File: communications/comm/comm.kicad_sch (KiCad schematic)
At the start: 2 parts, among them J1 Conn_Coaxial, U1 SX1276

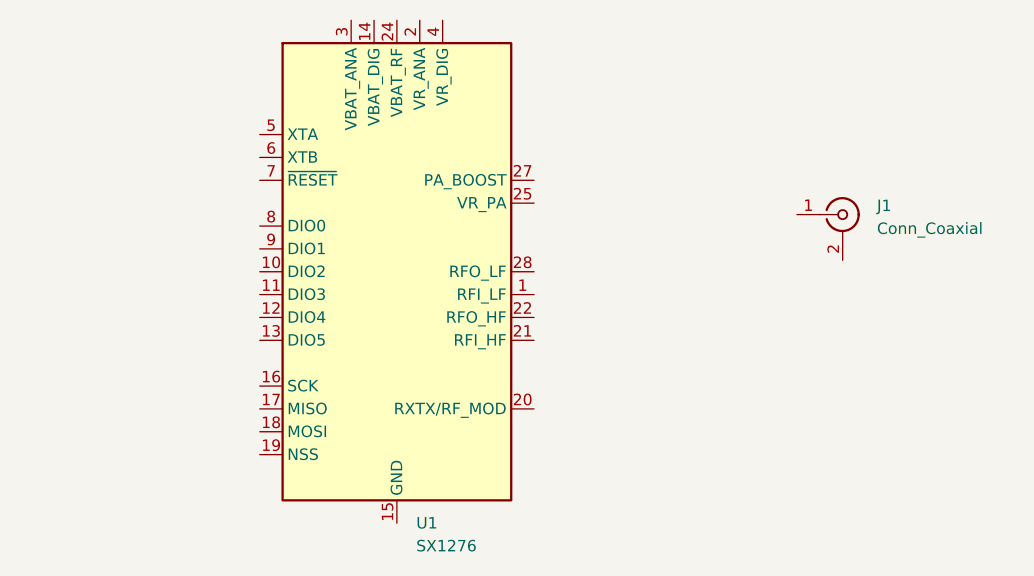
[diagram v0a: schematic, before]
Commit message: refresh
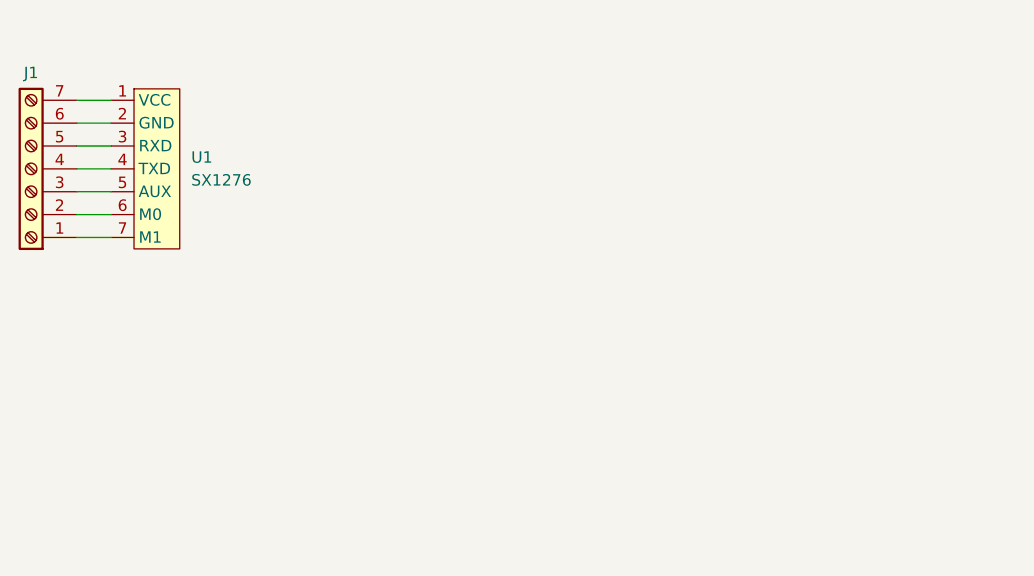
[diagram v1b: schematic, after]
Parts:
- removed J1: Conn_Coaxial, Connector_Coaxial:SMA_Molex_73251-1153_EdgeMount_Horizontal, symbol Connector:Conn_Coaxial
- removed U1: SX1276, Package_DFN_QFN:QFN-28-1EP_6x6mm_P0.65mm_EP4.8x4.8mm, symbol RF:SX1276
- added J1: Screw_Terminal_01x07, Connector_JST:JST_EH_B7B-EH-A_1x07_P2.50mm_Vertical, symbol Connector:Screw_Terminal_01x07
- added U1: SX1276, Connector_PinHeader_2.54mm:PinHeader_1x07_P2.54mm_Vertical, symbol me:SX1276-module
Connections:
- new net: J1.1 (Pin_1), U1.7 (M1)
- new net: J1.2 (Pin_2), U1.6 (M0)
- new net: J1.3 (Pin_3), U1.5 (AUX)
- new net: J1.4 (Pin_4), U1.4 (TXD)
- new net: J1.5 (Pin_5), U1.3 (RXD)
- new net: J1.6 (Pin_6), U1.2 (GND)
- new net: J1.7 (Pin_7), U1.1 (VCC)
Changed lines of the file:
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@@
 	(generator_version "9.0")
 	(paper "A4")
+	(wire
+		(pts
+			(xy 99.06 77.47) (xy 95.25 77.47)
+		)
+		(stroke
+			(width 0)
+			(type default)
+		)
+	)
+	(wire
+		(pts
+			(xy 99.06 87.63) (xy 95.25 87.63)
+		)
+		(stroke
+			(width 0)
+			(type default)
+		)
+	)
+	(wire
+		(pts
+			(xy 99.06 85.09) (xy 95.25 85.09)
+		)
+		(stroke
+			(width 0)
+			(type default)
+		)
+	)
+	(wire
+		(pts
+			(xy 99.06 82.55) (xy 95.25 82.55)
+		)
+		(stroke
+			(width 0)
+			(type default)
+		)
+	)
+	(wire
+		(pts
+			(xy 99.06 90.17) (xy 95.25 90.17)
+		)
+		(stroke
+			(width 0)
+			(type default)
+		)
+	)
+	(wire
+		(pts
+			(xy 99.06 80.01) (xy 95.25 80.01)
+		)
+		(stroke
+			(width 0)
+			(type default)
+		)
+	)
+	(wire
+		(pts
+			(xy 99.06 74.93) (xy 95.25 74.93)
+		)
+		(stroke
+			(width 0)
+			(type default)
+		)
+	)
 	(symbol
-		(lib_id "Connector:Conn_Coaxial")
-		(at 180.34 87.63 0)
+		(lib_id "Connector:Screw_Terminal_01x07")
+		(at 90.17 82.55 180)
 		(unit 1)
 		(exclude_from_sim no)
@@
 		(on_board yes)
 		(dnp no)
-		(fields_autoplaced yes)
 		(property "Reference" "J1"
-			(at 184.15 86.6531 0)
-			(effects
-				(font
-					(size 1.27 1.27)
-				)
-				(justify left)
-			)
-		)
-		(property "Value" "Conn_Coaxial"
-			(at 184.15 89.1931 0)
-			(effects
-				(font
-					(size 1.27 1.27)
-				)
-				(justify left)
-			)
-		)
-		(property "Footprint" "Connector_Coaxial:SMA_Molex_73251-1153_EdgeMount_Horizontal"
-			(at 180.34 87.63 0)
+			(at 90.17 71.882 0)
+			(effects
+				(font
+					(size 1.27 1.27)
+				)
+			)
+		)
+		(property "Value" "Screw_Terminal_01x07"
+			(at 90.17 71.12 0)
+			(effects
+				(font
+					(size 1.27 1.27)
+				)
+				(hide yes)
+			)
+		)
+		(property "Footprint" "Connector_JST:JST_EH_B7B-EH-A_1x07_P2.50mm_Vertical"
+			(at 90.17 82.55 0)
 			(effects
 				(font
@@
 		)
 		(property "Datasheet" "~"
-			(at 180.34 87.63 0)
-			(effects
-				(font
-					(size 1.27 1.27)
-				)
-				(hide yes)
-			)
-		)
-		(property "Description" "coaxial connector (BNC, SMA, SMB, SMC, Cinch/RCA, LEMO, ...)"
-			(at 180.34 87.63 0)
-			(effects
-				(font
-					(size 1.27 1.27)
-				)
-				(hide yes)
-			)
+			(at 90.17 82.55 0)
+			(effects
+				(font
+					(size 1.27 1.27)
+				)
+				(hide yes)
+			)
+		)
+		(property "Description" "Generic screw terminal, single row, 01x07, script generated (kicad-library-utils/schlib/autogen/connector/)"
+			(at 90.17 82.55 0)
+			(effects
+				(font
+					(size 1.27 1.27)
+				)
+				(hide yes)
+			)
+		)
+		(pin "3"
+		)
+		(pin "6"
+		)
+		(pin "5"
+		)
+		(pin "2"
+		)
+		(pin "4"
 		)
 		(pin "1"
 		)
-		(pin "2"
+		(pin "7"
 		)
 		(instances
@@
 	)
 	(symbol
-		(lib_id "RF:SX1276")
-		(at 130.81 93.98 0)
+		(lib_id "me:SX1276-module")
+		(at 104.14 82.55 0)
 		(unit 1)
 		(exclude_from_sim no)
@@
 		(fields_autoplaced yes)
 		(property "Reference" "U1"
-			(at 132.9533 121.92 0)
+			(at 107.95 81.2799 0)
 			(effects
 				(font
@@
 		)
 		(property "Value" "SX1276"
-			(at 132.9533 124.46 0)
+			(at 107.95 83.8199 0)
 			(effects
 				(font
@@
 			)
 		)
-		(property "Footprint" "Package_DFN_QFN:QFN-28-1EP_6x6mm_P0.65mm_EP4.8x4.8mm"
-			(at 130.81 101.6 0)
-			(effects
-				(font
-					(size 1.27 1.27)
-				)
-				(hide yes)
-			)
-		)
-		(property "Datasheet" "https://semtech.my.salesforce.com/sfc/p/#E0000000JelG/a/2R0000001Rbr/6EfVZUorrpoKFfvaF_Fkpgp5kzjiNyiAbqcpqh9qSjE"
-			(at 130.81 99.06 0)
-			(effects
-				(font
-					(size 1.27 1.27)
-				)
-				(hide yes)
-			)
-		)
-		(property "Description" "137 MHz to 1020 MHz Low Power Long Range Transceiver, spreading factor from 6 to 12, LoRA, QFN-28"
-			(at 130.81 93.98 0)
-			(effects
-				(font
-					(size 1.27 1.27)
-				)
-				(hide yes)
-			)
-		)
-		(pin "23"
-		)
-		(pin "16"
-		)
-		(pin "27"
+		(property "Footprint" "Connector_PinHeader_2.54mm:PinHeader_1x07_P2.54mm_Vertical"
+			(at 104.14 82.55 0)
+			(effects
+				(font
+					(size 1.27 1.27)
+				)
+				(hide yes)
+			)
+		)
+		(property "Datasheet" ""
+			(at 104.14 82.55 0)
+			(effects
+				(font
+					(size 1.27 1.27)
+				)
+				(hide yes)
+			)
+		)
+		(property "Description" ""
+			(at 104.14 82.55 0)
+			(effects
+				(font
+					(size 1.27 1.27)
+				)
+				(hide yes)
+			)
+		)
+		(pin "2"
+		)
+		(pin "7"
+		)
+		(pin "4"
 		)
 		(pin "3"
 		)
-		(pin "12"
-		)
-		(pin "9"
-		)
-		(pin "7"
-		)
-		(pin "14"
+		(pin "5"
 		)
 		(pin "6"
 		)
-		(pin "10"
-		)
-		(pin "5"
-		)
-		(pin "8"
-		)
-		(pin "13"
-		)
 		(pin "1"
 		)
-		(pin "25"
-		)
-		(pin "24"
-		)
-		(pin "28"
-		)
-		(pin "18"
-		)
-		(pin "19"
-		)
-		(pin "2"
-		)
-		(pin "20"
-		)
-		(pin "17"
-		)
-		(pin "15"
-		)
-		(pin "22"
-		)
-		(pin "21"
-		)
-		(pin "11"
-		)
-		(pin "26"
-		)
-		(pin "29"
-		)
-		(pin "4"
-		)
 		(instances
